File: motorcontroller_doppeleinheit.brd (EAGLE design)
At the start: 160 x 100 mm, 21 parts

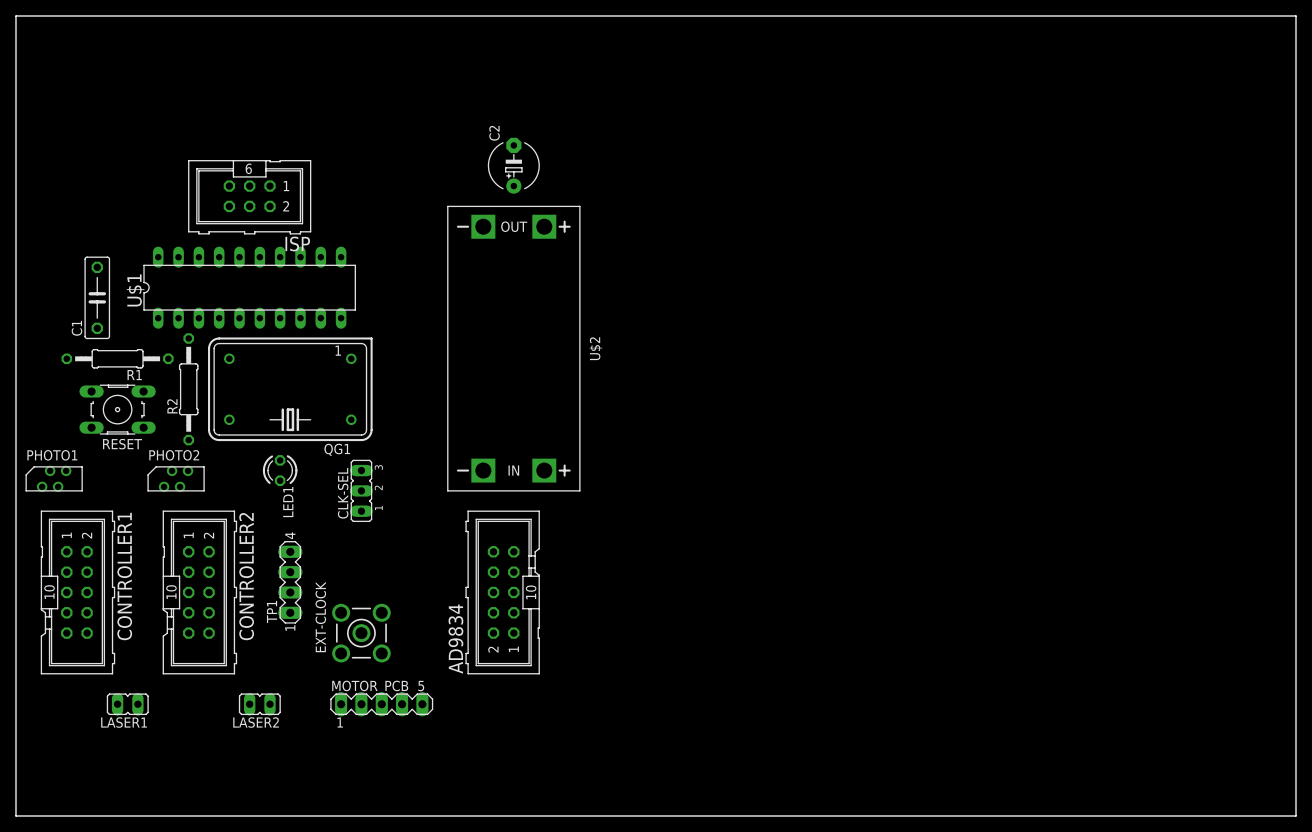
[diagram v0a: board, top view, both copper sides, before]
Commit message: ...
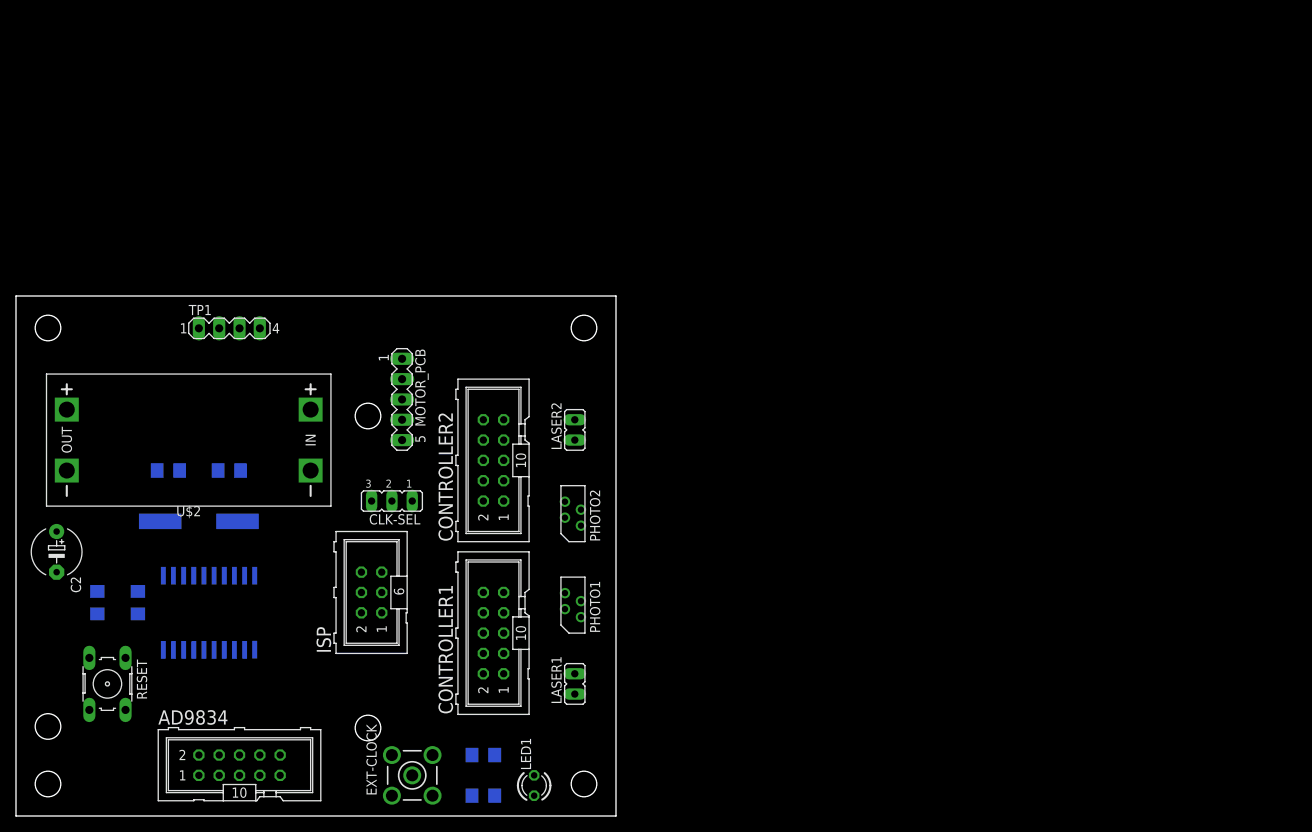
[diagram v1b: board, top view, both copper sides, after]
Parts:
- removed QG1: 16,384Mhz, crystal:DIL14S
- added C3, C4: 22pF, rcl:C1206
- added Q1: 16,384Mhz, crystal:HC49UP
- added R3: 10k, rcl:R1206
- C1: device rcl:C075-032X103 -> rcl:C1206
- R1: device rcl:0207/12 -> rcl:C1206
- R2: device rcl:0207/12 -> rcl:R1206
- U$1: value TINY2313-*P* -> TINY2313-*S*; device avr-7:DIL20 -> avr-7:SO20L$
- moved C2 74.8 mm to (5.08, 33.0), turned to 270 degrees
- moved PHOTO1 72.1 mm to (71.1, 22.9), turned to 90 degrees
- moved R2 62.7 mm to (58.4, 2.54), flipped to the bottom, turned to 0 degrees
- moved LASER1 55.9 mm to (69.8, 16.5), turned to 0 degrees
- moved PHOTO2 55.0 mm to (71.1, 34.3), turned to 90 degrees
- moved CONTROLLER1 52.3 mm to (59.7, 22.9), turned to 90 degrees
- moved LASER2 52.2 mm to (69.8, 48.3), turned to 0 degrees
- moved ISP 51.8 mm to (44.5, 27.9), turned to 90 degrees
- moved LED1 50.6 mm to (64.8, 3.81), turned to 90 degrees
- moved U$2 42.2 mm to (21.6, 47.0), turned to 0 degrees
- moved U$1 41.0 mm to (24.1, 25.4), flipped to the bottom, turned to 180 degrees
- moved CONTROLLER2 40.4 mm to (59.7, 44.5), turned to 90 degrees
- moved AD9834 39.5 mm to (27.9, 6.35), turned to 0 degrees
- moved MOTOR_PCB 38.2 mm to (48.3, 52.1), turned to 270 degrees
- moved C1 38.1 mm to (10.2, 26.7), flipped to the bottom, turned to 270 degrees
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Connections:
- new net N$5: C3.2, Q1.2, U$1.4
- net +5V: now also R3.2; no longer QG1.14
- net GND: now also C3.1, C4.1; no longer QG1.7
- net LOCKED: now also R3.1
- net N$1: now also C4.2, Q1.1; no longer QG1.8
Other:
- board size 160 x 100 mm -> 75 x 65 mm
